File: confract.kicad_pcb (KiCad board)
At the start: 2 copper layers, 44 parts, among them J1 Conn_01x05, J10 GS2, J11 Conn_01x04, J12 GS2, J13 GS2, J14 GS2, J15 GS2, J16 Conn_01x02, J2 GS3, J3 Conn_01x05, J4 GS3, J5 Audio-Jack-4, J6 GS2, J7 GS2, J8 GS2, J9 GS3, Q1 Q_NMOS_GSD, SW1 SW_Push, SW10 SW_Push, SW11 SW_Push, SW12 SW_Push, SW13 SW_Push, SW14 SW_Push, SW15 SW_Push, SW16 SW_Push, SW17 SW_Push, SW2 SW_Push, SW3 SW_Push, SW4 SW_Push, SW5 SW_Push, SW6 SW_Push, SW7 SW_Push, SW8 SW_Push, SW9 SW_Push, U1 MCP23017_QFN

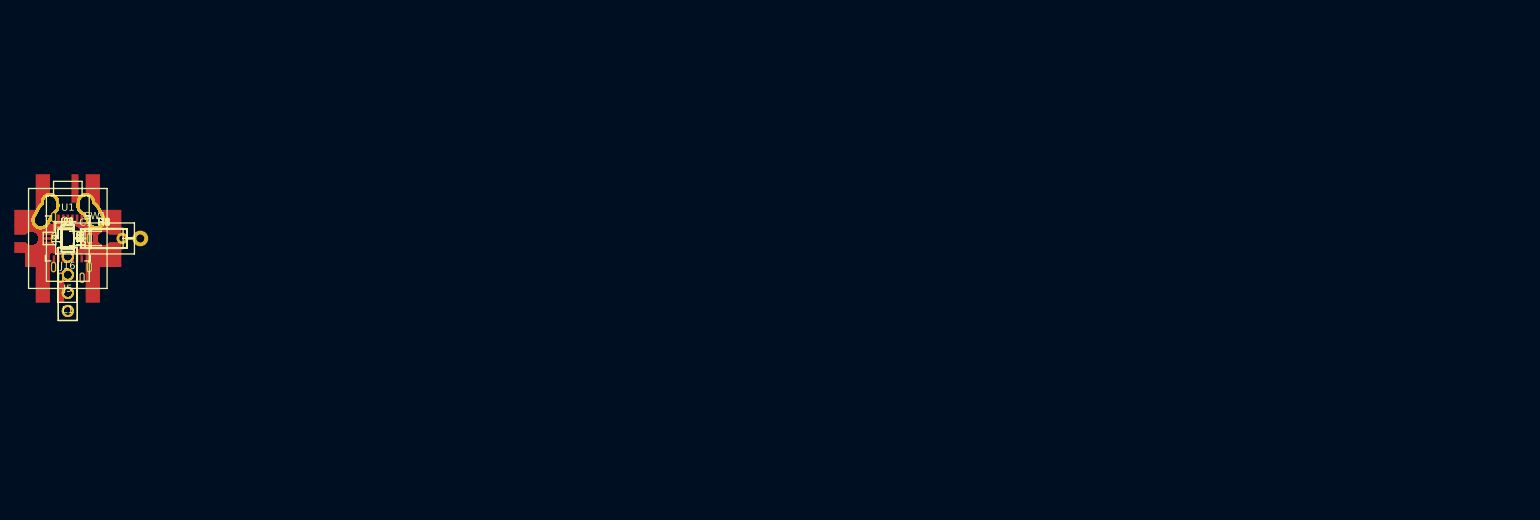
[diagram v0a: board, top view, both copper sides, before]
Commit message: load pcb-outline
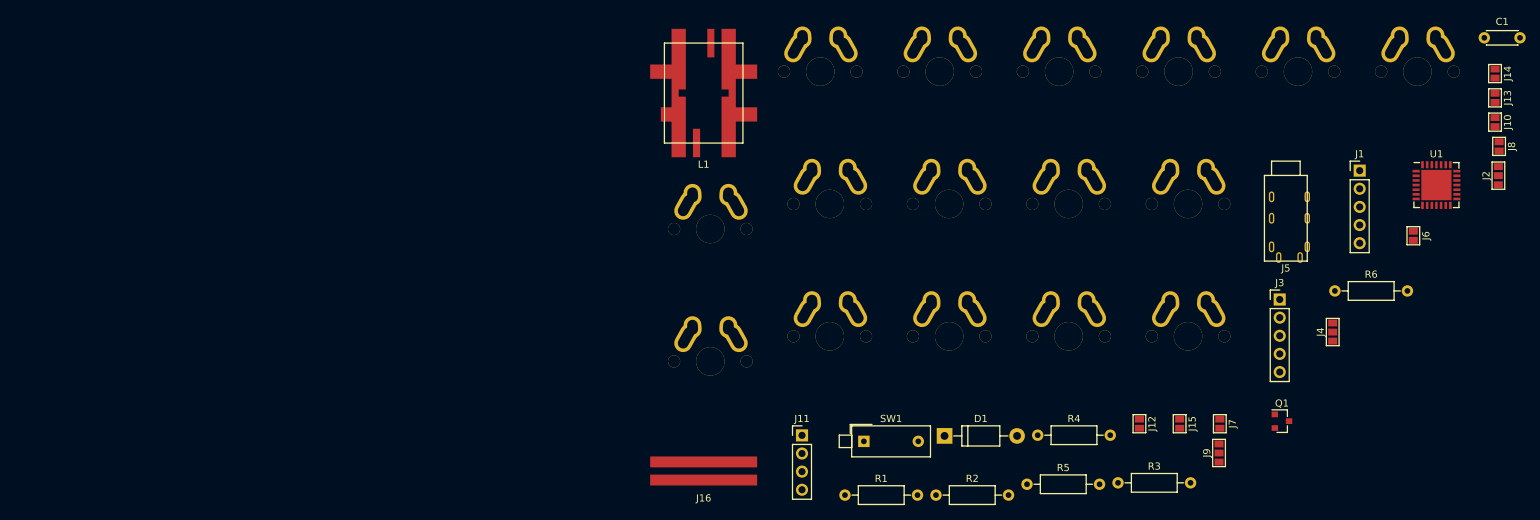
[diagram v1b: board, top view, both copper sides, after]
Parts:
- moved J14 201.3 mm to (339.5, 76.8)
- moved J8 200.9 mm to (340.1, 87.0)
- moved J13 200.9 mm to (339.5, 80.2)
- moved J10 200.6 mm to (339.5, 83.6)
- moved J2 200.6 mm to (340.0, 91.1)
- moved C1 200.4 mm to (338.0, 71.8)
- moved U1 191.9 mm to (331.3, 92.4)
- moved SW2 190.5 mm to (328.7, 76.6)
- moved J6 188.5 mm to (328.1, 99.5)
- moved J1 181.2 mm to (320.6, 90.4)
- moved J4 177.7 mm to (316.8, 113.0)
- moved R6 177.6 mm to (317.1, 107.3)
- moved SW4 173.9 mm to (311.9, 76.6)
- moved Q1 172.0 mm to (309.7, 125.5)
- moved J5 170.6 mm to (310.2, 97.1)
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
